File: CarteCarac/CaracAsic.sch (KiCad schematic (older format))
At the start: 2 parts

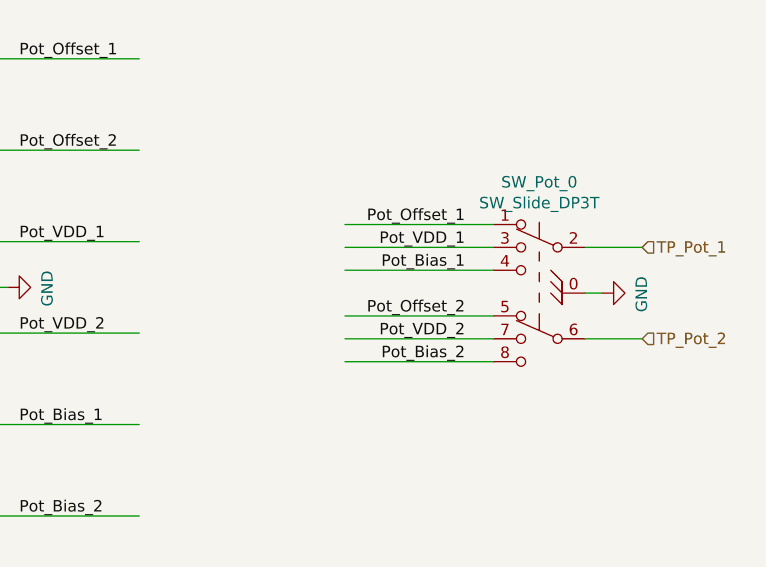
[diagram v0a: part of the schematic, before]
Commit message: Routé, verif pre-envoie
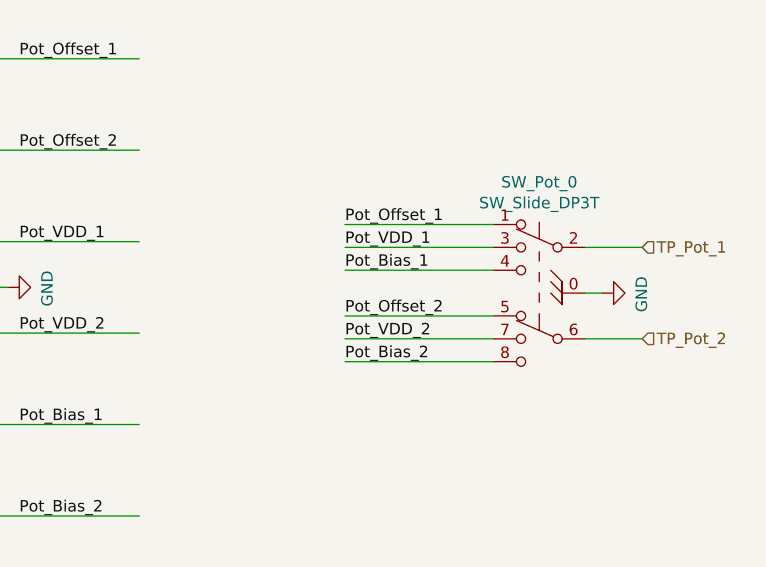
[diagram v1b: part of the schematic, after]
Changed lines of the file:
@@
 F15 "-R34" I R 2900 3875 50
 $EndSheet
-Text Label 9050 2325 2    50   ~ 0
+Text Label 8525 2325 0    50   ~ 0
 Pot_Offset_1
 Wire Wire Line
@@
 Wire Wire Line
 	9175 2725 8525 2725
-Text Label 9050 2425 2    50   ~ 0
+Text Label 8525 2425 0    50   ~ 0
 Pot_VDD_1
-Text Label 9050 2525 2    50   ~ 0
+Text Label 8525 2525 0    50   ~ 0
 Pot_Bias_1
-Text Label 9050 2725 2    50   ~ 0
+Text Label 8525 2725 0    50   ~ 0
 Pot_Offset_2
-Text Label 9050 2825 2    50   ~ 0
+Text Label 8525 2825 0    50   ~ 0
 Pot_VDD_2
-Text Label 9050 2925 2    50   ~ 0
+Text Label 8525 2925 0    50   ~ 0
 Pot_Bias_2
 Text Label 7100 1600 0    50   ~ 0
